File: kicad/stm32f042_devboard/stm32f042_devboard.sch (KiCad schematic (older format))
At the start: 18 parts, among them J1 USB_B_Micro, J2 Conn_01x04, J3 Conn_01x09, J4 Conn_01x03, J5 Conn_01x03, J6 Conn_01x03, SW1 SW_Push, U1 STM32F042F6Px, U2 AMS1117-3.3

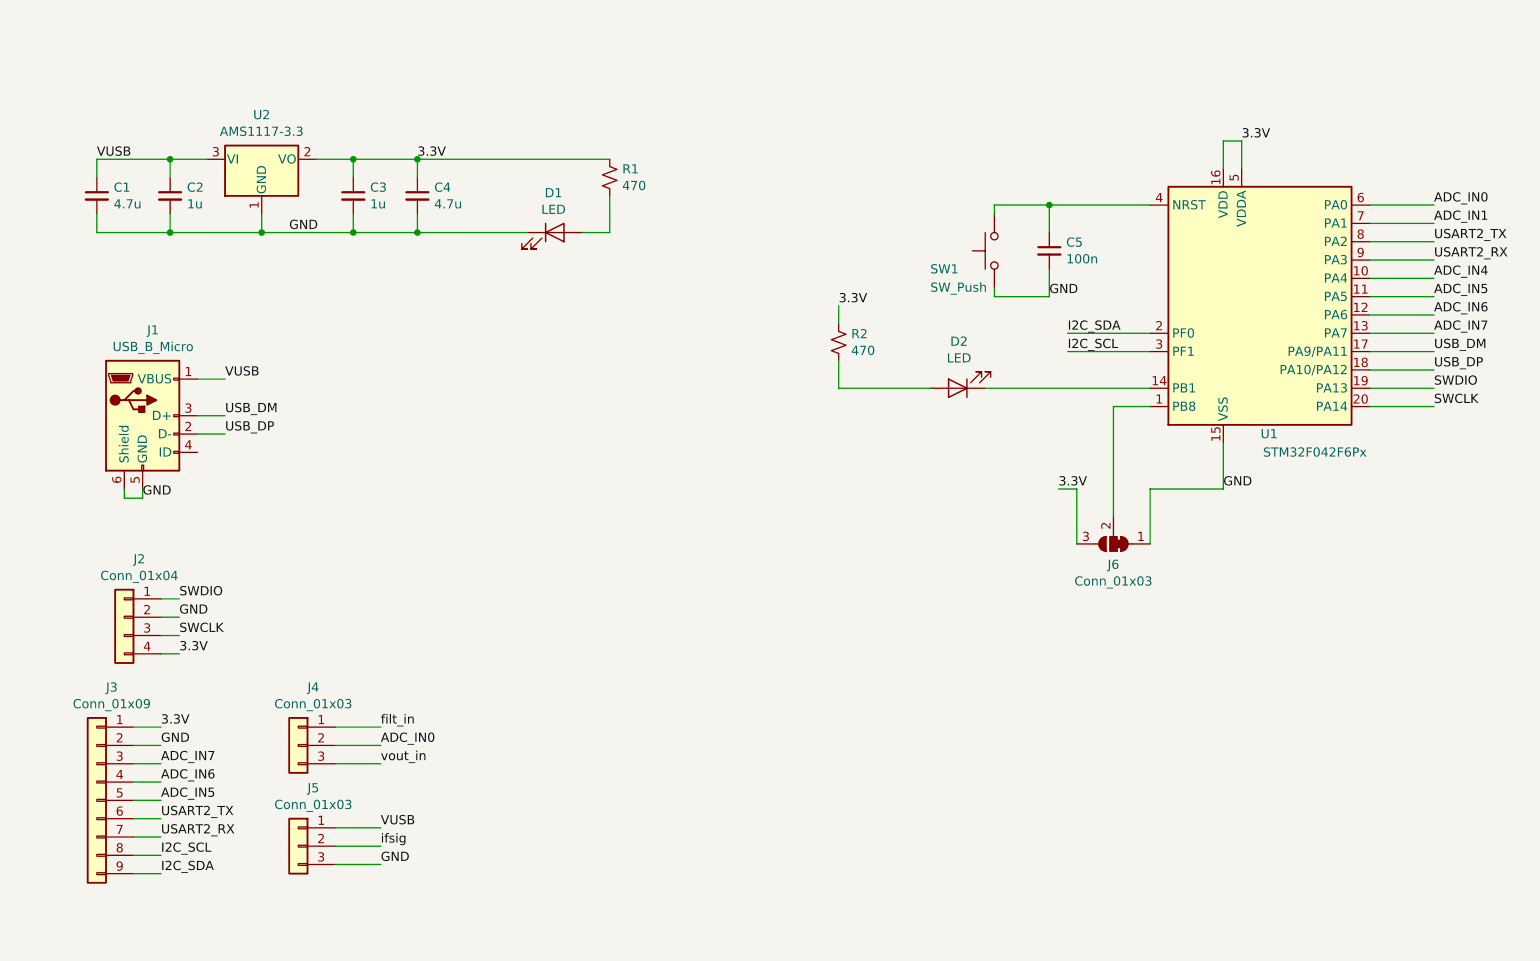
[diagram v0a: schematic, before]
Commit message: updated
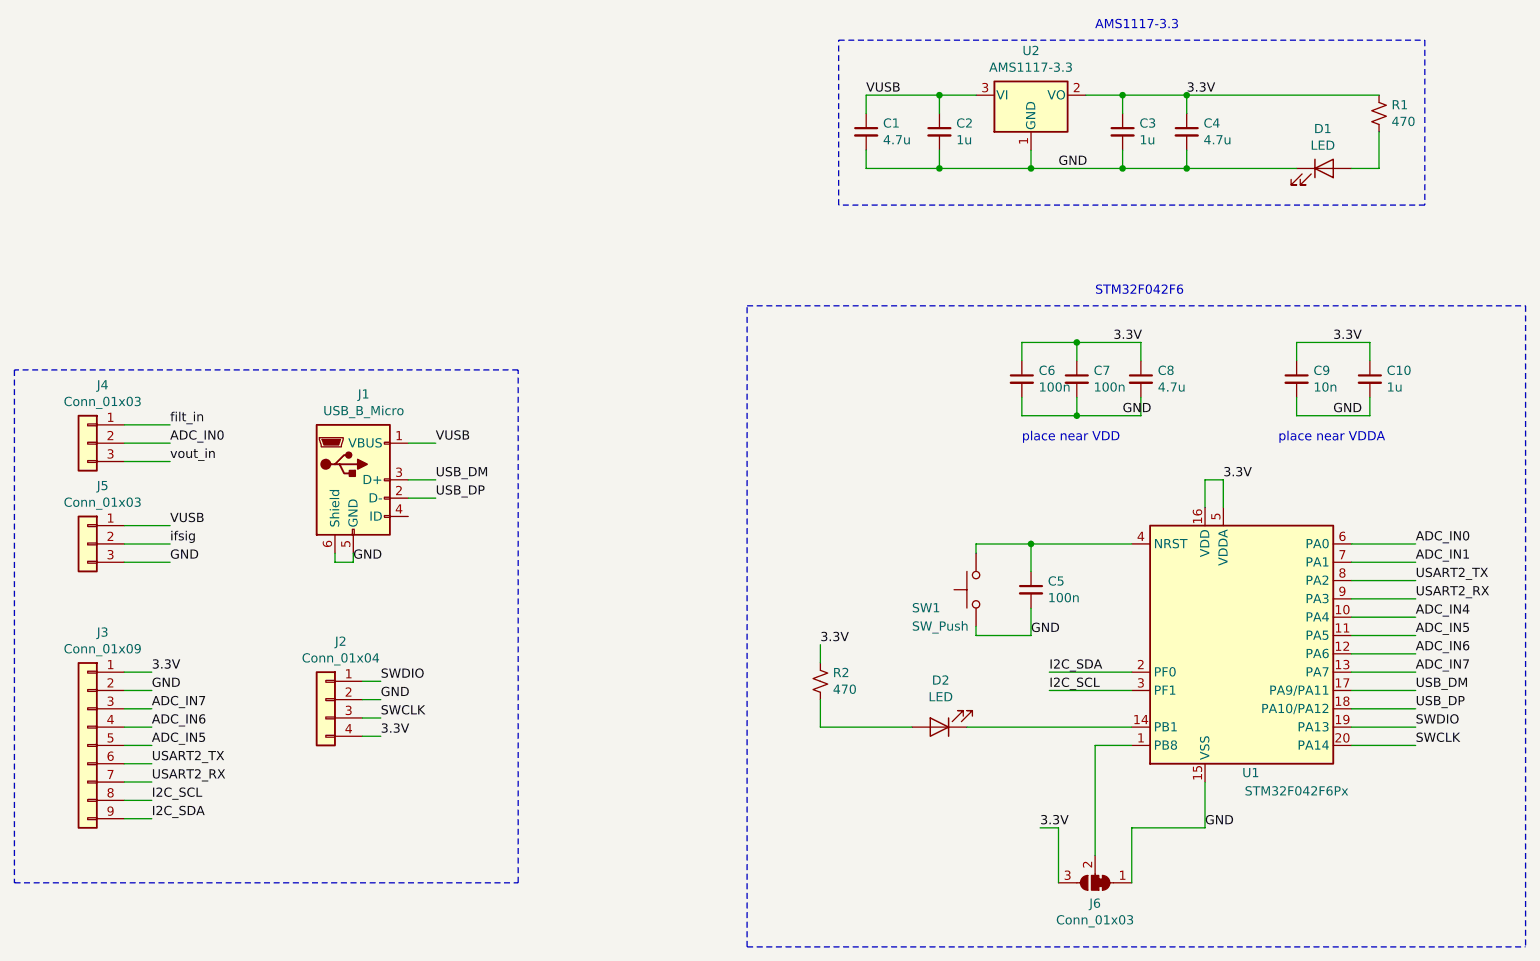
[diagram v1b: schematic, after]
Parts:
- added C10: 1u, Capacitor_SMD:C_0805_2012Metric_Pad1.15x1.40mm_HandSolder, symbol Device:C_Small
- added C6, C7: 100n, Capacitor_SMD:C_0805_2012Metric_Pad1.15x1.40mm_HandSolder, symbol Device:C_Small
- added C8: 4.7u, Capacitor_SMD:C_0805_2012Metric_Pad1.15x1.40mm_HandSolder, symbol Device:C_Small
- added C9: 10n, Capacitor_SMD:C_0805_2012Metric_Pad1.15x1.40mm_HandSolder, symbol Device:C_Small
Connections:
- net 3.3V: now also C10.1, C6.1, C7.1, C8.1, C9.1
- net GND: now also C10.2, C6.2, C7.2, C8.2, C9.2
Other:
- note added: "AMS1117-3.3"
- note added: "STM32F042F6"
- note added: "place near VDD"
- note added: "place near VDDA"
- moved on the sheet: C1, C2, C3, C4, C5, D1, D2, J1, J2, J3, J4, J5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
